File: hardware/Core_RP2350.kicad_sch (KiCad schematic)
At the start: 69 parts, among them J1 5-146281-3, J2 5-146281-3, J3 AudioJack3, J4 USB_C_Receptacle_USB2.0, J5 Micro_SD_Card_Det_Hirose_DM3AT, SW2 SPST-NO, U2 W25Q16JVUXIQ, U3 ADUM4160, U32 RP2350_80QFN

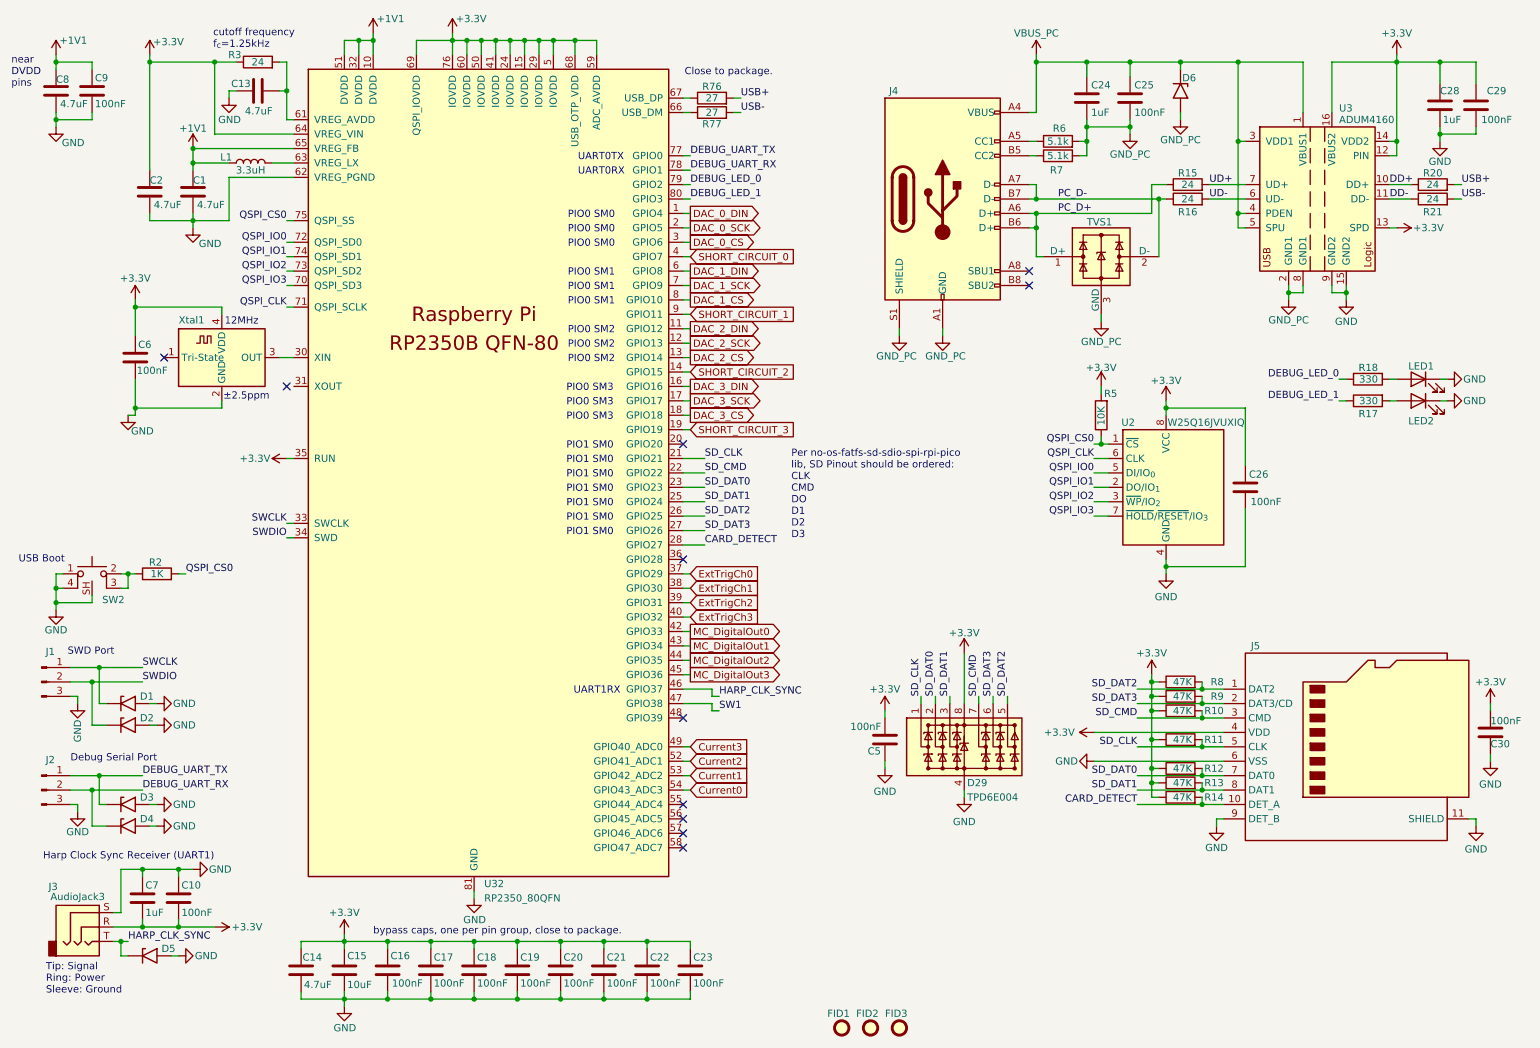
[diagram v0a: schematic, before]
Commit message: update bom
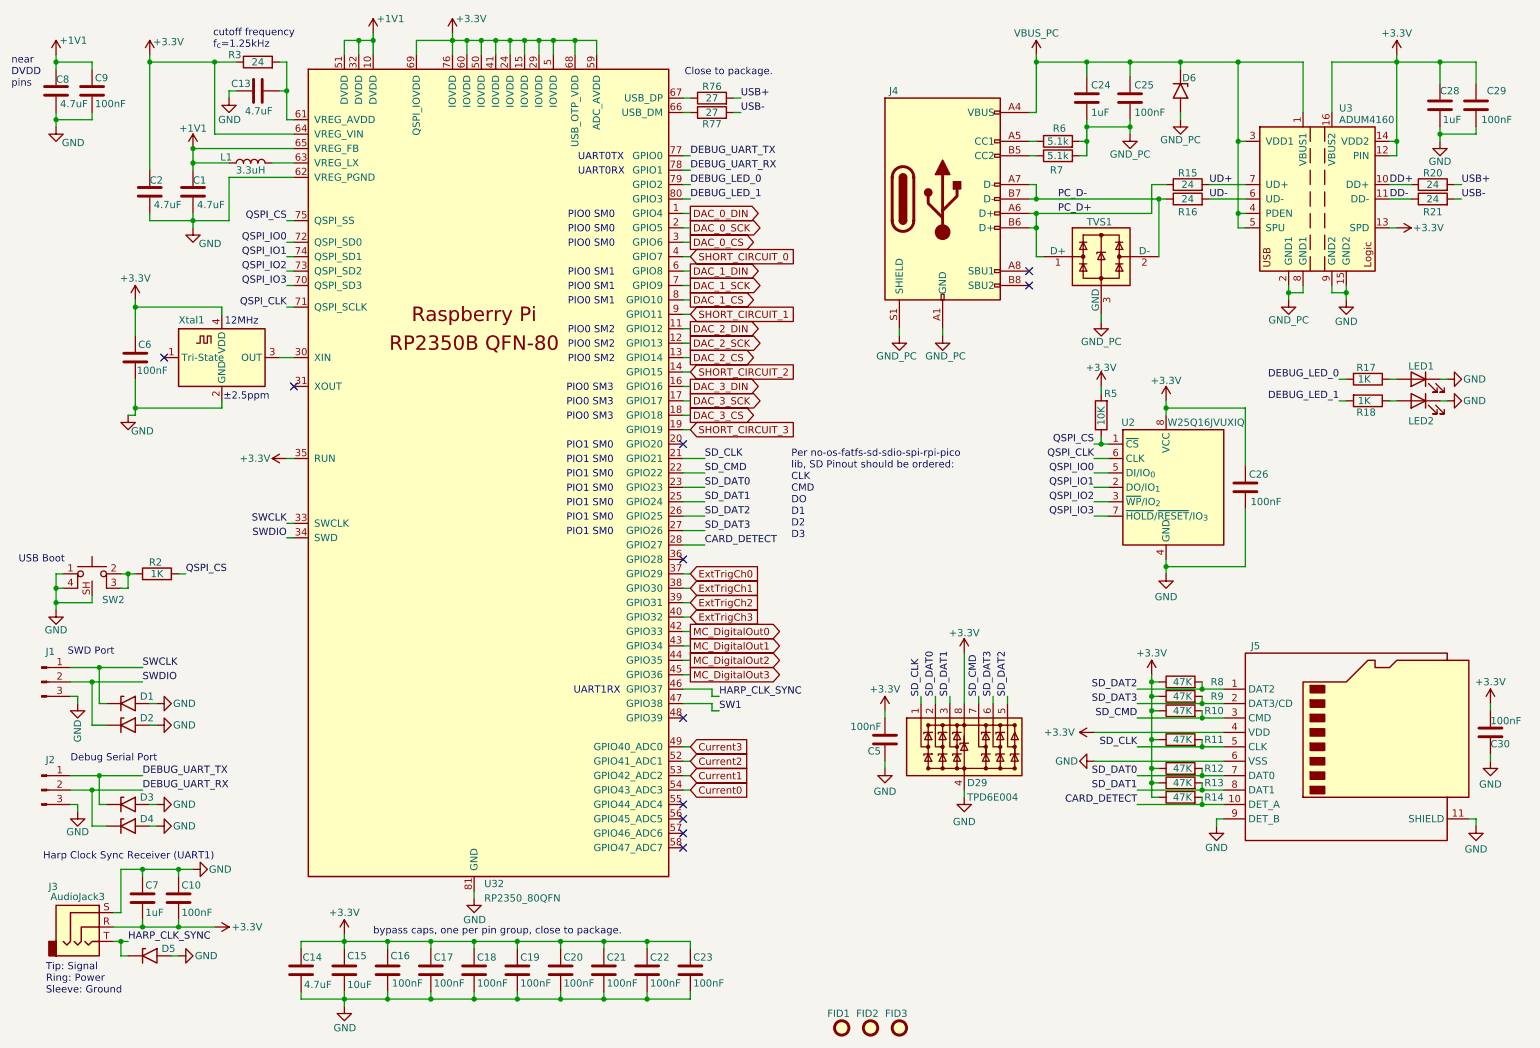
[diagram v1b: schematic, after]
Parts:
- removed R17, R18: 330, Resistor_SMD:R_0603_1608Metric, symbol harp.device.quad.dac:R_0603
- added R17, R18: 1K, Resistor_SMD:R_0402_1005Metric, symbol Device:R
- R10, R11, R12, R13, R14, R8, R9: Link (none) -> https://www.digikey.com/en/products/detail/yageo/RC0402FR-0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; Manufacturer (none) -> YAGEO; Manufacturer Number (none) -> RC0402FR-0747KL
- R2: Link (none) -> https://www.digikey.com/en/products/detail/panasonic-electr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; Manufacturer (none) -> Panasonic Electronic Components; Manufacturer Number (none) -> ERJ-2RKF1001X
- R5: Link (none) -> https://www.digikey.com/en/products/detail/samsung-electro-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; Manufacturer (none) -> Samsung Electro-Mechanics; Manufacturer Number (none) -> RC1005F103CS
- R6, R7: Link (none) -> https://www.digikey.com/en/products/detail/yageo/RC0402FR-0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; Manufacturer (none) -> YAGEO; Manufacturer Number (none) -> RC0402FR-075K1L
- SW2: Manufacturer Number (none) -> 435451019820
- U32: Link (none) -> https://www.digikey.com/en/products/detail/raspberry-pi/SC1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; Manufacturer (none) -> Raspberry Pi; Manufacturer Number (none) -> SC1510-A4
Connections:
- net DEBUG_LED_0: now also R17.2
- net DEBUG_LED_1: now also R18.2
- net at LED1.2 (A): now also R18.1
- net at LED2.2 (A): now also R17.1
- net QSPI_CS0 renamed QSPI_CS

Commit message: update bom
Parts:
- J1, J2: Alternate n/a -> (none); Link n/a -> https://www.digikey.com/en/products/detail/te-connectivity-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; Manufacturer n/a -> TE Connectivity AMP Connectors; Manufacturer Number n/a -> 5-146281-3; Notes DNP -> (none)
